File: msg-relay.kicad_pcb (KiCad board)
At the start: 2 copper layers, 100 x 100 mm, 29 parts, among them J1 Screw_Terminal_01x02, J2 Conn_01x03_Male, J3 Conn_01x03_Male, J4 Conn_01x03_Male, J5 Conn_01x03_Male, J6 Screw_Terminal_01x02, K1 SANYOU_SRD_Form_C, K2 SANYOU_SRD_Form_C, K3 SANYOU_SRD_Form_C, K4 SANYOU_SRD_Form_C, Q1 BC847, Q2 BC847, Q3 BC847, Q4 BC847

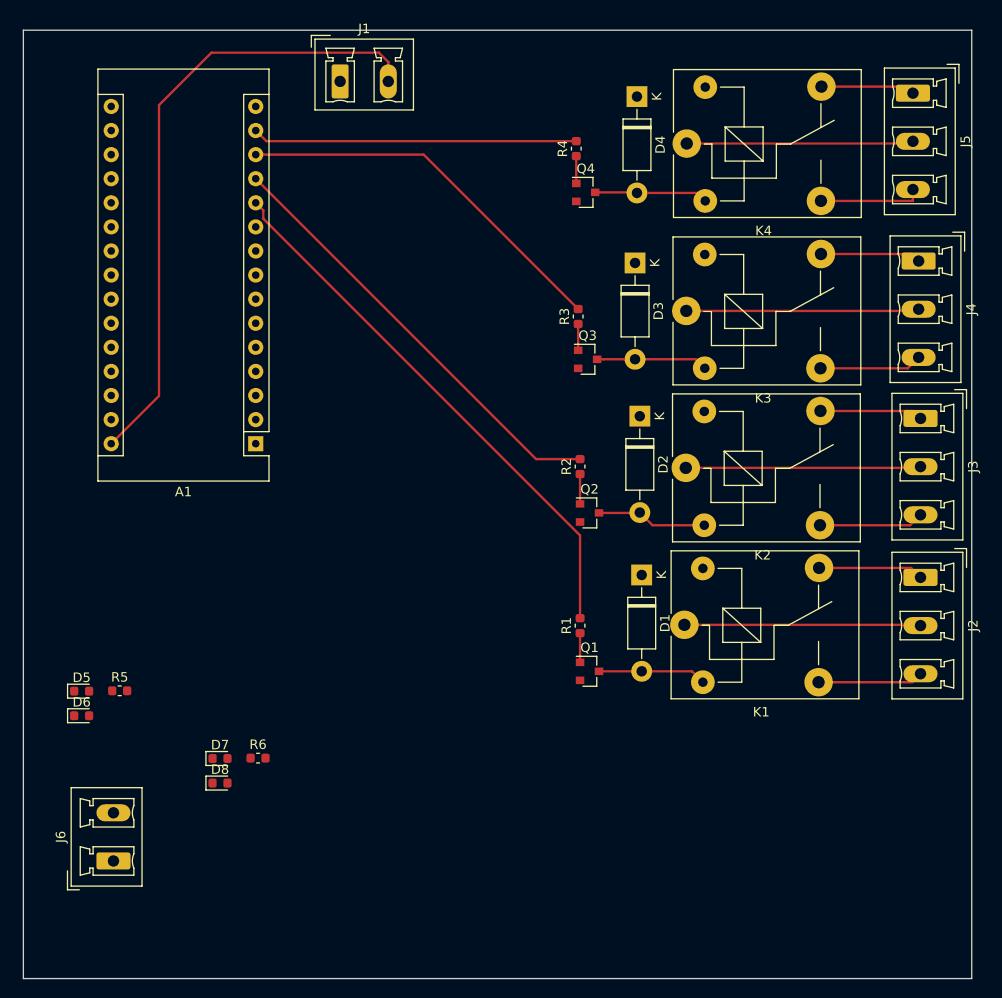
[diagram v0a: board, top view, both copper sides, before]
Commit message: Made v01
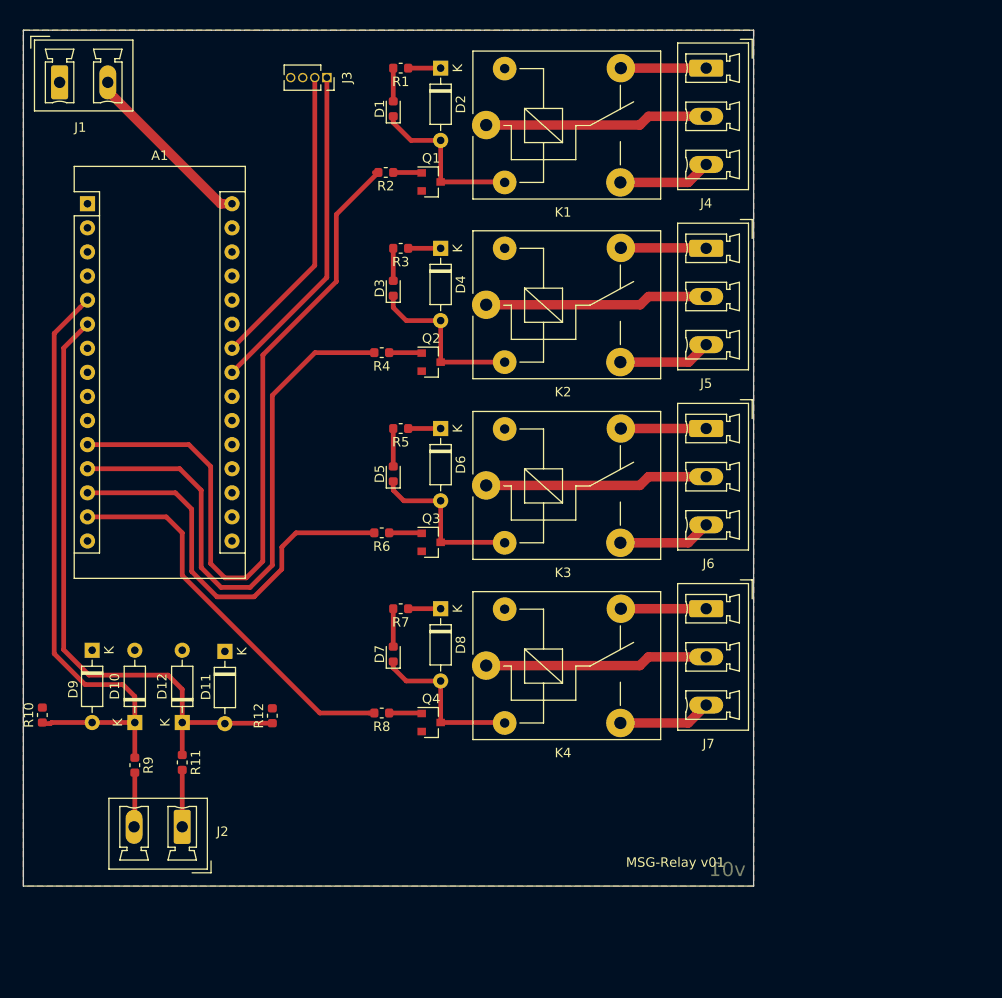
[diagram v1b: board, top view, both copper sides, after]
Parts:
- added D10: BAT43, Diode_THT:D_DO-35_SOD27_P7.62mm_Horizontal, F.Cu at (91.8, 123.0)
- added D11: BAT43, Diode_THT:D_DO-35_SOD27_P7.62mm_Horizontal, F.Cu at (101.2, 115.5)
- added D12: BAT43, Diode_THT:D_DO-35_SOD27_P7.62mm_Horizontal, F.Cu at (96.8, 123.0)
- added D9: BAT43, Diode_THT:D_DO-35_SOD27_P7.62mm_Horizontal, F.Cu at (87.2, 115.4)
- added J7: Conn_01x03_Male, Connector_Phoenix_MC_HighVoltage:PhoenixContact_MCV_1,5_3-G-5.08_1x03_P5.08mm_Vertical, F.Cu at (152.0, 111.0)
- added R10: 10k, Resistor_SMD:R_0603_1608Metric, F.Cu at (82.0, 122.2)
- added R11: 10k, Resistor_SMD:R_0603_1608Metric, F.Cu at (96.8, 127.2)
- added R12: 10k, Resistor_SMD:R_0603_1608Metric, F.Cu at (106.2, 122.3)
- added R7: 1k, Resistor_SMD:R_0603_1608Metric, F.Cu at (119.8, 111.0)
- added R8: 10k, Resistor_SMD:R_0603_1608Metric, F.Cu at (117.8, 122.0)
- added R9: 10k, Resistor_SMD:R_0603_1608Metric, F.Cu at (91.8, 127.5)
- D1, D3: value 1N4007 -> LED; footprint Diode_THT:D_DO-41_SOD81_P10.16mm_Horizontal -> LED_SMD:LED_0603_1608Metric
- D2, D4: value 1N4007 -> 1N4148; footprint Diode_THT:D_DO-41_SOD81_P10.16mm_Horizontal -> Diode_THT:D_DO-35_SOD27_P7.62mm_Horizontal
- D5, D7: value D -> LED; footprint Diode_SMD:D_0603_1608Metric -> LED_SMD:LED_0603_1608Metric
- D6, D8: value D -> 1N4148; footprint Diode_SMD:D_0603_1608Metric -> Diode_THT:D_DO-35_SOD27_P7.62mm_Horizontal
- J2: value Conn_01x03_Male -> Screw_Terminal_01x02; footprint Connector_Phoenix_MC_HighVoltage:PhoenixContact_MCV_1,5_3-G-5.08_1x03_P5.08mm_Vertical -> Connector_Phoenix_MC_HighVoltage:PhoenixContact_MCV_1,5_2-G-5.08_1x02_P5.08mm_Vertical
- J3: value Conn_01x03_Male -> Conn_01x04; footprint Connector_Phoenix_MC_HighVoltage:PhoenixContact_MCV_1,5_3-G-5.08_1x03_P5.08mm_Vertical -> Connector_PinSocket_1.27mm:PinSocket_1x04_P1.27mm_Vertical
- J6: value Screw_Terminal_01x02 -> Conn_01x03_Male; footprint Connector_Phoenix_MC_HighVoltage:PhoenixContact_MCV_1,5_2-G-5.08_1x02_P5.08mm_Vertical -> Connector_Phoenix_MC_HighVoltage:PhoenixContact_MCV_1,5_3-G-5.08_1x03_P5.08mm_Vertical
- R1, R3, R5: value R -> 1k
- R2, R4, R6: value R -> 10k
- moved J2 82.2 mm to (96.8, 134.0), turned to 180 degrees
- moved J6 77.4 mm to (152.0, 92.0), turned to 270 degrees
- moved J3 72.2 mm to (112.0, 55.0)
- moved R1 61.8 mm to (119.8, 54.0), turned to 180 degrees
- moved K4 59.0 mm to (128.8, 117.0)
- moved Q4 58.2 mm to (123.0, 123.0)
- moved K1 56.7 mm to (128.8, 60.0)
- moved D1 55.7 mm to (119.0, 58.3), turned to 90 degrees
- moved Q1 54.2 mm to (123.0, 66.0)
- moved D6 48.5 mm to (124.0, 92.0), turned to 270 degrees
- moved D2 42.3 mm to (124.0, 54.0)
- moved R5 40.5 mm to (119.8, 92.0), turned to 180 degrees
- moved D5 40.1 mm to (119.0, 96.8), turned to 90 degrees
- moved R2 37.2 mm to (118.2, 65.0), turned to 180 degrees
- moved A1 30.9 mm to (86.8, 68.3), turned to 0 degrees
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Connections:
- A1 pad 23: Net-(A1-Pad23) -> SDA
- A1 pad 24: Net-(A1-Pad24) -> SCL
- D1 pad 1: +5V -> Net-(D1-Pad1)
- D2 pad 2: Net-(D2-Pad2) -> Net-(D1-Pad1)
- D3 pad 1: +5V -> Net-(D3-Pad1)
- D4 pad 2: Net-(D4-Pad2) -> Net-(D3-Pad1)
- D5 pad 1: +5V -> Net-(D5-Pad1)
- D5 pad 2: /Input1/OUT -> Net-(D5-Pad2)
- D6 pad 1: /Input1/OUT -> +5V
- D6 pad 2: GND -> Net-(D5-Pad1)
- D7 pad 1: +5V -> Net-(D7-Pad1)
- D7 pad 2: /Input2/OUT -> Net-(D7-Pad2)
- D8 pad 1: /Input2/OUT -> +5V
- D8 pad 2: GND -> Net-(D7-Pad1)
- J2 pad 1: Net-(J2-Pad1) -> INPUT2
- J2 pad 2: Net-(J2-Pad2) -> INPUT1
- J3 pad 1: Net-(J3-Pad1) -> SDA
- J3 pad 2: Net-(J3-Pad2) -> SCL
- J3 pad 3: Net-(J3-Pad3) -> +5V
- J6 pad 1: INPUT2 -> Net-(J6-Pad1)
- J6 pad 2: INPUT1 -> Net-(J6-Pad2)
- K1 pad 1: Net-(J2-Pad2) -> Net-(J4-Pad2)
- K1 pad 2: Net-(D1-Pad2) -> Net-(D1-Pad1)
- K1 pad 3: Net-(J2-Pad3) -> Net-(J4-Pad3)
- K1 pad 4: Net-(J2-Pad1) -> Net-(J4-Pad1)
- K2 pad 1: Net-(J3-Pad2) -> Net-(J5-Pad2)
- K2 pad 2: Net-(D2-Pad2) -> Net-(D3-Pad1)
- K2 pad 3: Net-(J3-Pad3) -> Net-(J5-Pad3)
- K2 pad 4: Net-(J3-Pad1) -> Net-(J5-Pad1)
- K3 pad 1: Net-(J4-Pad2) -> Net-(J6-Pad2)
- K3 pad 2: Net-(D3-Pad2) -> Net-(D5-Pad1)
- K3 pad 3: Net-(J4-Pad3) -> Net-(J6-Pad3)
- K3 pad 4: Net-(J4-Pad1) -> Net-(J6-Pad1)
- K4 pad 1: Net-(J5-Pad2) -> Net-(J7-Pad2)
- K4 pad 2: Net-(D4-Pad2) -> Net-(D7-Pad1)
- K4 pad 3: Net-(J5-Pad3) -> Net-(J7-Pad3)
- K4 pad 4: Net-(J5-Pad1) -> Net-(J7-Pad1)
- Q1 pad 3: Net-(D1-Pad2) -> Net-(D1-Pad1)
- Q2 pad 3: Net-(D2-Pad2) -> Net-(D3-Pad1)
- Q3 pad 3: Net-(D3-Pad2) -> Net-(D5-Pad1)
- Q4 pad 3: Net-(D4-Pad2) -> Net-(D7-Pad1)
- R1 pad 1: Net-(Q1-Pad1) -> +5V
- R1 pad 2: RELAY1 -> Net-(D1-Pad2)
- R2 pad 1: Net-(Q2-Pad1) -> Net-(Q1-Pad1)
- R2 pad 2: RELAY2 -> RELAY1
- R3 pad 1: Net-(Q3-Pad1) -> +5V
- R3 pad 2: RELAY3 -> Net-(D3-Pad2)
- R4 pad 1: Net-(Q4-Pad1) -> Net-(Q2-Pad1)
- R4 pad 2: RELAY4 -> RELAY2
- R5 pad 1: /Input1/OUT -> +5V
- R5 pad 2: INPUT1 -> Net-(D5-Pad2)
- R6 pad 1: /Input2/OUT -> Net-(Q3-Pad1)
- R6 pad 2: INPUT2 -> RELAY3
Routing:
- net /Input2/OUT: track 0.00 -> 66.1 mm
- net /Input1/OUT: track 0.00 -> 65.4 mm
- net +12V: track 66.7 -> 18.9 mm
- net SDA: track 0.00 -> 35.2 mm
- net SCL: track 0.00 -> 32.2 mm
- net Net-(J2-Pad2): track 24.9 -> 0.00 mm
- net Net-(J3-Pad2): track 24.8 -> 0.00 mm
- net Net-(J7-Pad2): track 0.00 -> 23.6 mm
- net Net-(J6-Pad2): track 0.00 -> 23.6 mm
- net RELAY1: track 58.0 -> 77.5 mm
- net Net-(D3-Pad1): track 0.00 -> 17.9 mm
- net Net-(D1-Pad1): track 0.00 -> 17.6 mm
- net Net-(D5-Pad1): track 0.00 -> 17.5 mm
- net Net-(D7-Pad1): track 0.00 -> 17.4 mm
- net RELAY2: track 46.4 -> 61.0 mm
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- added copper zone on B.Cu, net +5V
- added copper zone on F.Cu, net GND
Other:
- board size 100 x 100 mm -> 77 x 90.2 mm
- net class Default: trace_width 0.25 -> 0.5
- net class Power added: clearance 0.2, trace_width 1, via_dia 0.8, via_drill 0.4
- rule pad_to_mask_clearance: 0.051 -> 0.05
- rule solder_mask_min_width: 0.25 -> 0.3
- rule trace_min: 0.2 -> 0.5
- rule via_min_drill: 0.3 -> 0.4
- rule via_min_size: 0.4 -> 0.8
- board text added: "MSG-Relay v01"
- board text added: "v01"
